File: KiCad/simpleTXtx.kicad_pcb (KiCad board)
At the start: 2 copper layers, 18 x 30 mm, 13 parts, among them J1 BAT, J2 VIDEO, Q1 2SC1815

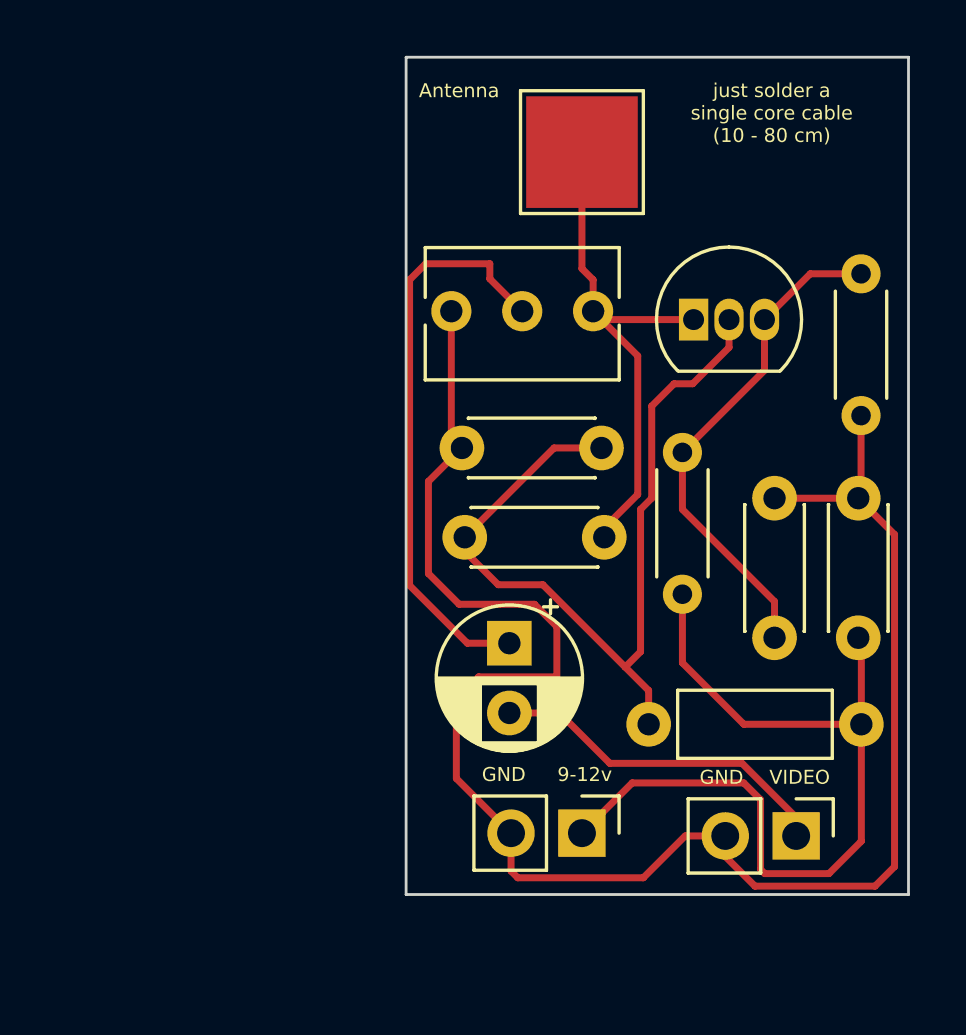
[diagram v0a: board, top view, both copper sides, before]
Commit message: update project
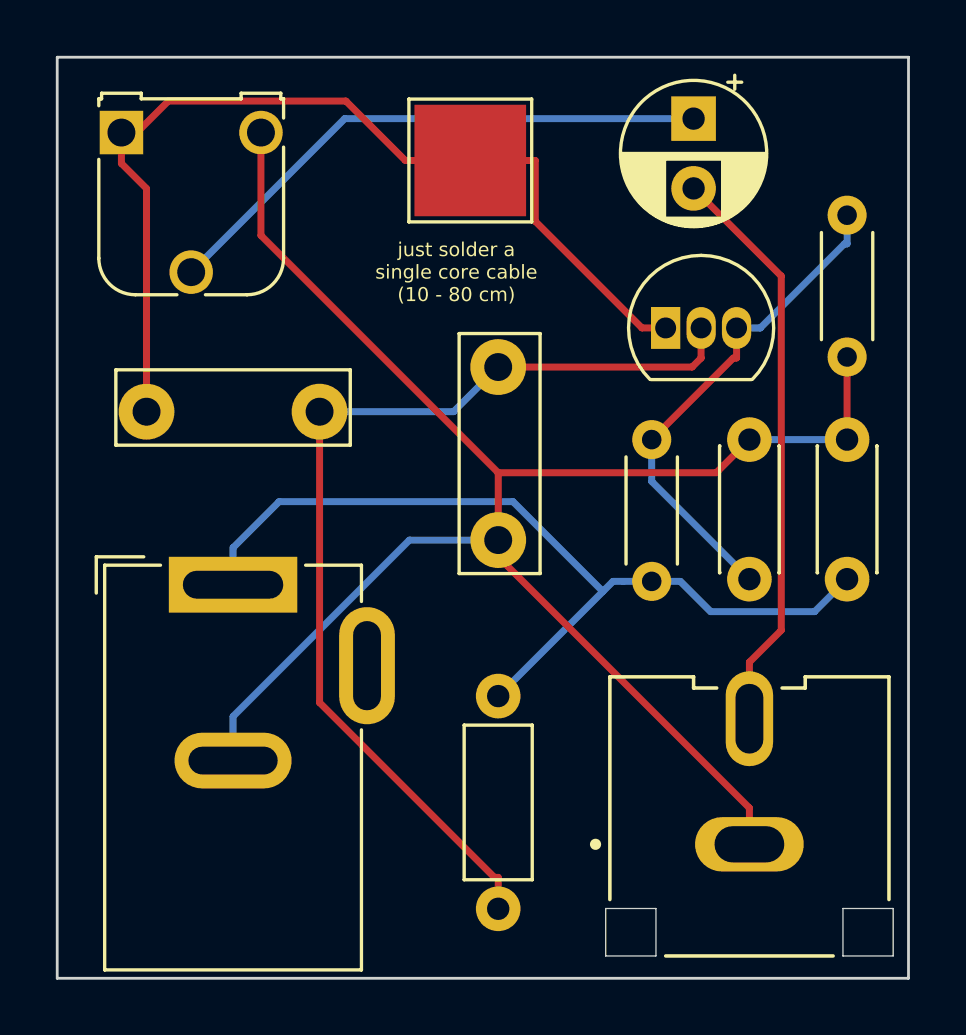
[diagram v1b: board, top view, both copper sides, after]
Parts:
- removed J1: BAT, Connector_PinHeader_2.54mm:PinHeader_1x02_P2.54mm_Vertical
- added J3: RCJ-044, RCJ-044:CUI_RCJ-044, F.Cu at (157.0, 85.0)
- C3, C4: footprint Capacitor_THT:C_Disc_D4.3mm_W1.9mm_P5.00mm -> Capacitor_THT:C_Disc_D11.0mm_W5.0mm_P5.00mm
- J2: value VIDEO -> Barrel_Jack_MountingPin; footprint Connector_PinHeader_2.54mm:PinHeader_1x02_P2.54mm_Vertical -> Connector_BarrelJack:BarrelJack_GCT_DCJ200-10-A_Horizontal
- RV1: footprint Potentiometer_THT:Potentiometer_Bourns_3266Y_Vertical -> Potentiometer_THT:Potentiometer_Runtron_RM-065_Vertical
- moved J2 22.1 mm to (138.5, 75.7), turned to 0 degrees
- moved C5 19.9 mm to (155.0, 59.0)
- moved RV1 18.1 mm to (134.5, 59.5)
- moved C4 16.4 mm to (136.0, 69.5), turned to 0 degrees
- moved L1 13.0 mm to (148.0, 79.7), turned to -90 degrees
- moved C3 4.41 mm to (148.0, 68.4), turned to -90 degrees
- moved AE1 4.01 mm to (147.0, 60.5)
- moved C2 2.28 mm to (157.0, 70.5)
- moved R1 2.16 mm to (160.5, 67.5)
- moved C1 2.14 mm to (160.5, 70.5)
- moved R2 1.19 mm to (153.5, 70.5)
- moved Q1 1.04 mm to (154.0, 66.5)
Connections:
- C5 pad 2: Net-(J2-Pad1) -> Net-(C5-Pad2)
- J2 pad 1: Net-(J2-Pad1) -> Net-(C1-Pad2)
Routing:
- net Net-(C5-Pad2): track 0.00 -> 20.8 mm
- net Net-(AE1-A): track 18.8 -> 35.2 mm
- net Net-(J2-Pad1): track 12.5 -> 0.00 mm
- net Net-(Q1-C): track 30.8 -> 36.1 mm
- net GND: track 63.8 -> 62.4 mm
- net Net-(C1-Pad2): track 31.2 -> 31.7 mm
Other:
- board size 18 x 30 mm -> 30.5 x 33 mm
- board text removed: "9-12v"
- board text removed: "Antenna"
- board text removed: "GND"
- board text removed: "VIDEO"
